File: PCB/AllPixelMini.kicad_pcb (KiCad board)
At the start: 2 copper layers, 58.4 x 14.2 mm, 25 parts, among them CON1 ML_USB_MINI, CON2 BARREL_JACK, P1 CONN_1, P2 CONN_1, Q1 NPN, U1 ATMEGA16U4/32U4, Y1 16MHz

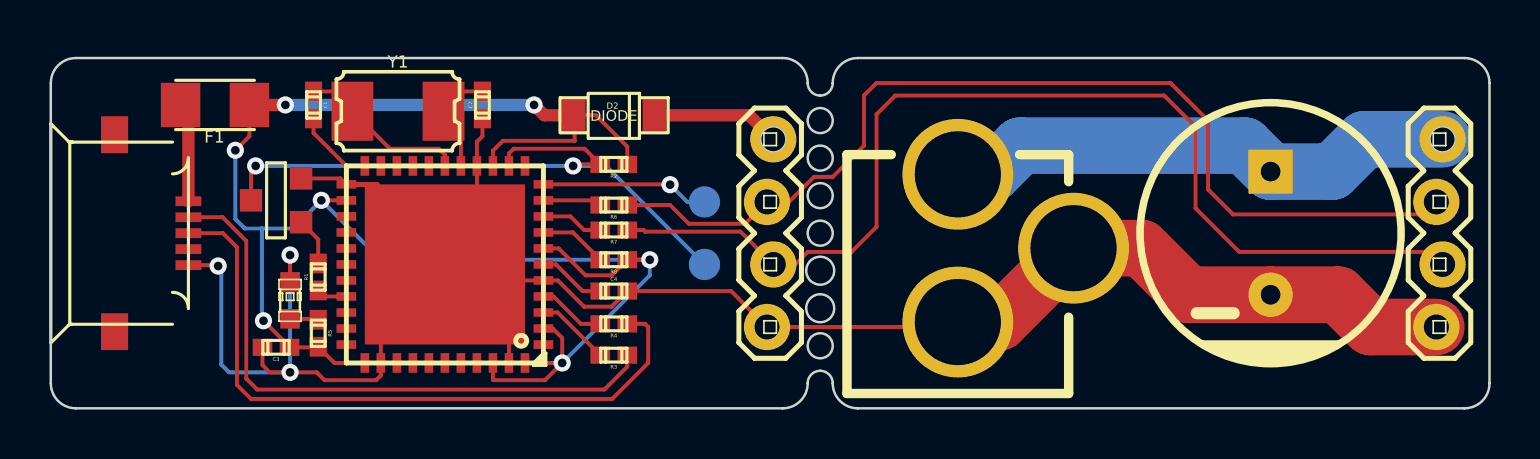
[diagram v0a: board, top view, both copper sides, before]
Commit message: tweaked mini layout
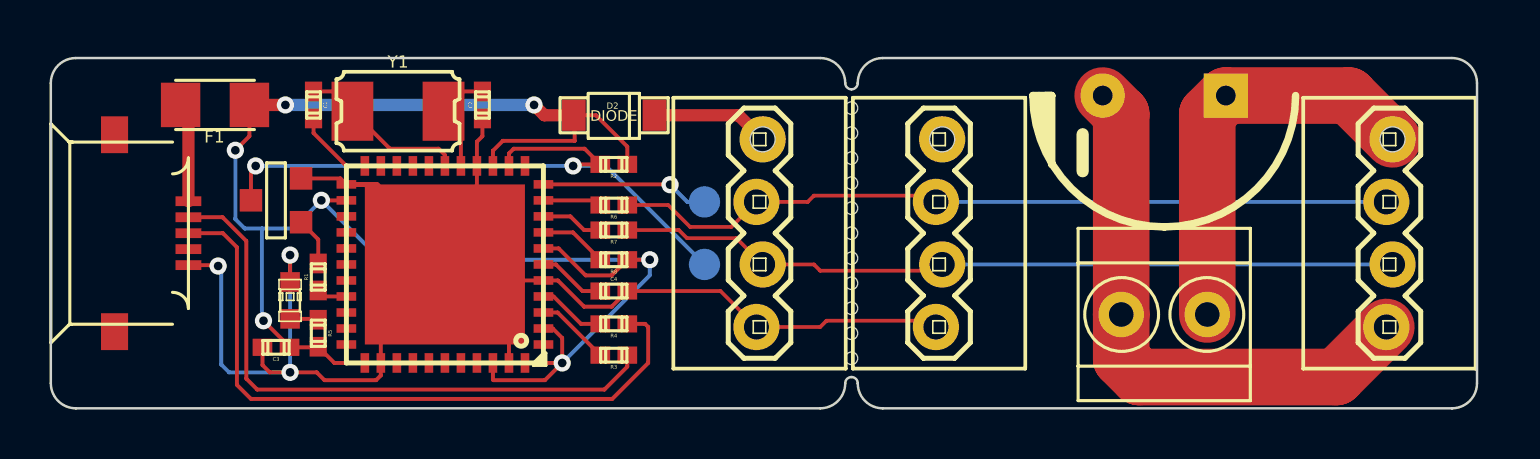
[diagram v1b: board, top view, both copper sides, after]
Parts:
- removed CON2: BARREL_JACK, ML_BARREL_JACK_ROUND_PADS_SHORT_3_5mmHoles
- added 20mil_drill: VAL**, 20mil_drill, F.Cu at (140.2, 36.6)
- added 20mil_drill: VAL**, 20mil_drill, F.Cu at (140.2, 45.7)
- added 20mil_drill: VAL**, 20mil_drill, F.Cu at (140.2, 46.7)
- added 20mil_drill: VAL**, 20mil_drill, F.Cu at (140.2, 37.6)
- added 20mil_drill: VAL**, 20mil_drill, F.Cu at (140.2, 38.6)
- added 20mil_drill: VAL**, 20mil_drill, F.Cu at (140.2, 43.7)
- added 20mil_drill: VAL**, 20mil_drill, F.Cu at (140.2, 39.6)
- added 20mil_drill: VAL**, 20mil_drill, F.Cu at (140.2, 40.6)
- added 20mil_drill: VAL**, 20mil_drill, F.Cu at (140.2, 41.7)
- added 20mil_drill: VAL**, 20mil_drill, F.Cu at (140.2, 42.7)
- added 20mil_drill: VAL**, 20mil_drill, F.Cu at (140.2, 44.7)
- added JP3: PT_INPUT, ML_SparkFun-1X04_LOCK_SCREW, F.Cu at (143.8, 41.7)
- added P3: CONN_2, 2P-3.5, F.Cu at (152.9, 45.0)
- C5: footprint CP_10x12.5mm -> CP_10x12.5mm_Half
- JP1: value OUTPUT2 -> PT_OUTPUT; footprint 4-Pin-Lock -> ML_SparkFun-1X04_LOCK_SCREW
- JP2: footprint 4-Pin-Lock -> ML_SparkFun-1X04_LOCK_SCREW
- moved C5 7.06 mm to (152.9, 36.1), turned to 90 degrees
- moved JP1 2.03 mm to (162.1, 41.7)
- moved JP2 0.43 mm to (136.5, 41.7)
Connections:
- U1 pad 45: GND -> (no net)
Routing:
- net CLK: track 44.0 -> 31.9 mm
- net DATA: track 40.8 -> 31.8 mm
- net VJACK: track 21.1 -> 16.7 mm
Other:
- board size 58.4 x 14.2 mm -> 57.9 x 14.2 mm
